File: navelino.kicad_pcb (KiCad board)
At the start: 2 copper layers, 45.6 x 37.3 mm, 71 parts, among them CON1 USB-MINI-B, IC1 ATMEGA328P-A, P1 CONN_5X2, P3 CONN_6, SW0 SW_PUSH, SW1 SMD-SWITCH-TACTILE-SPST-NO(4P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, SW2 SMD-SWITCH-TACTILE-SPST-NO(4P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, U1 XC6204B332MR, X0 CRYSTAL

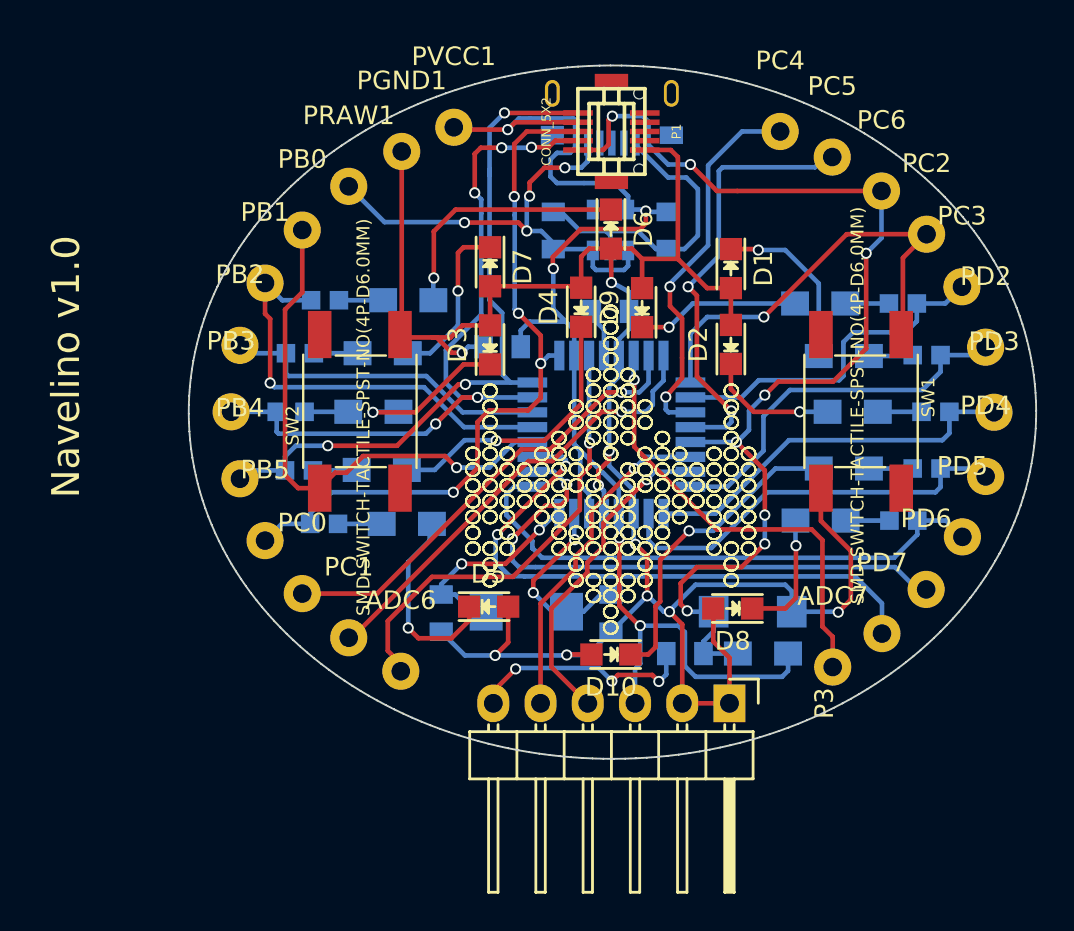
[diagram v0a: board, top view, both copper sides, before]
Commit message: Un poco de amor para el Silkscreen
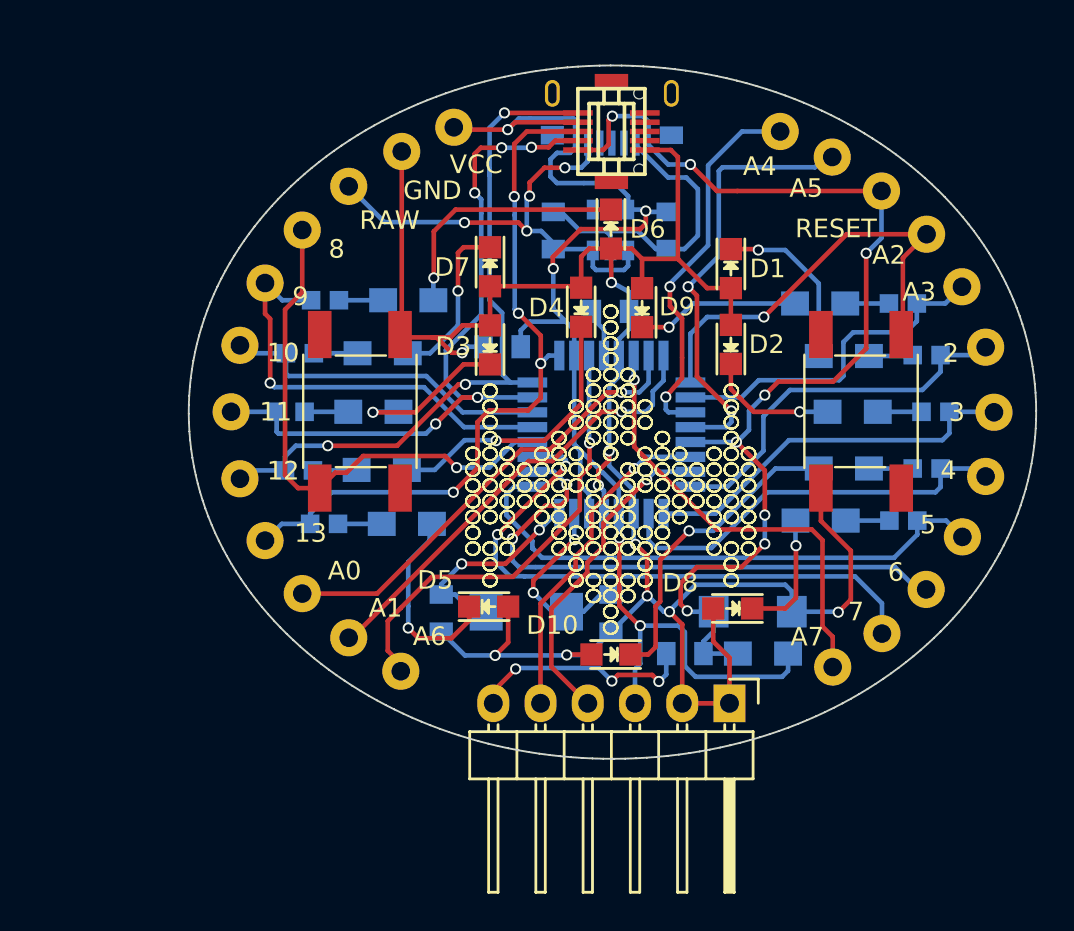
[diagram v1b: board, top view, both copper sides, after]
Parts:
- CON1: value USB-MINI-B -> USB
- renumbered PB2 to 10, PB3 to 11, PB4 to 12, PB5 to 13, PD2 to 2, PD3 to 3, PD4 to 4, PD5 to 5, PD6 to 6, PD7 to 7, PB0 to 8, PB1 to 9, PC0 to A0, PC1 to A1, PC2 to A2, PC3 to A3, PC4 to A4, PC5 to A5, ADC6 to A6, ADC7 to A7, PGND1 to GND, PRAW1 to RAW, PC6 to RESET, PVCC1 to VCC
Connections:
- CON1 pad 6: Net-(CON1-Pad6) -> (no net)
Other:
- board text added: "Hacker SpaceVLC"
